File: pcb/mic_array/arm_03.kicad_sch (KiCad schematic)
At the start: 16 parts, among them U25 IM72D128V01XTMA1, U26 IM72D128V01XTMA1, U27 IM72D128V01XTMA1, U28 IM72D128V01XTMA1, U29 IM72D128V01XTMA1, U30 IM72D128V01XTMA1, U31 IM72D128V01XTMA1, U32 IM72D128V01XTMA1

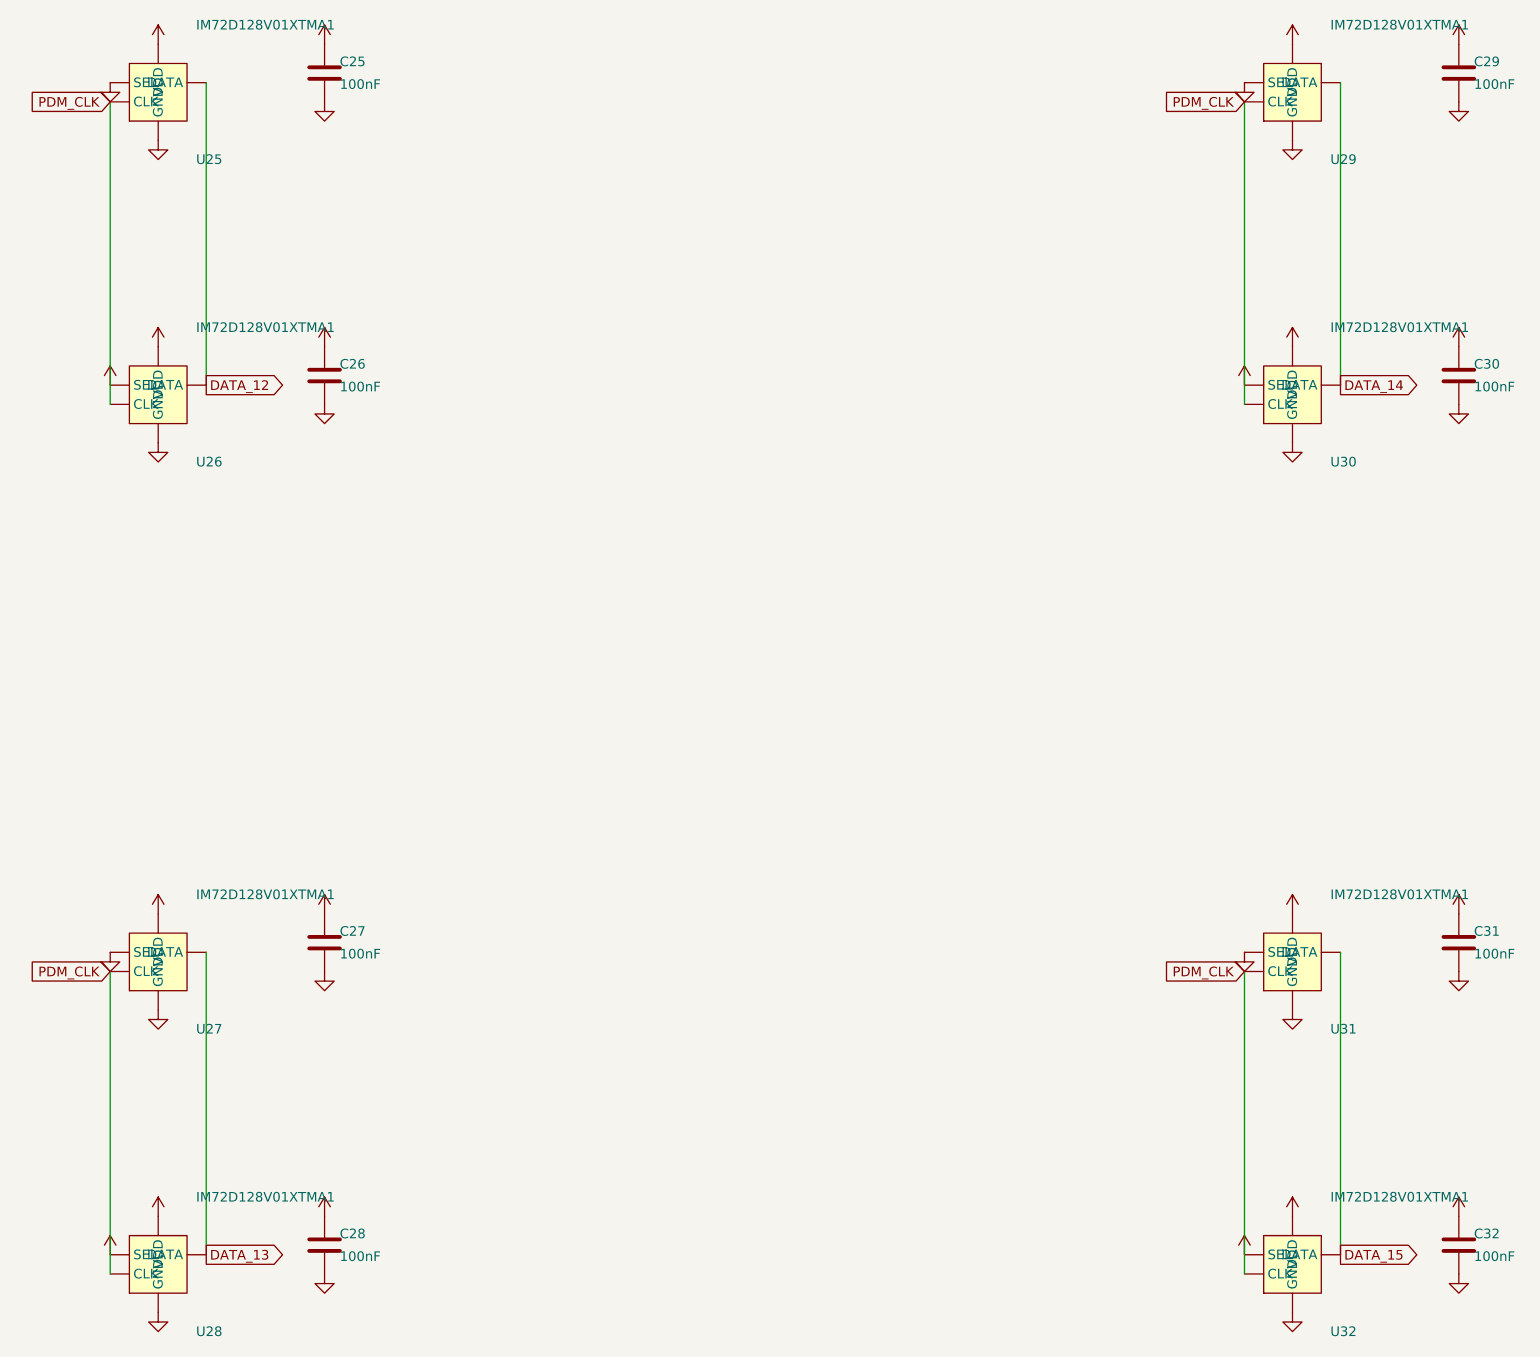
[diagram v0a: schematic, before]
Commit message: Updated.
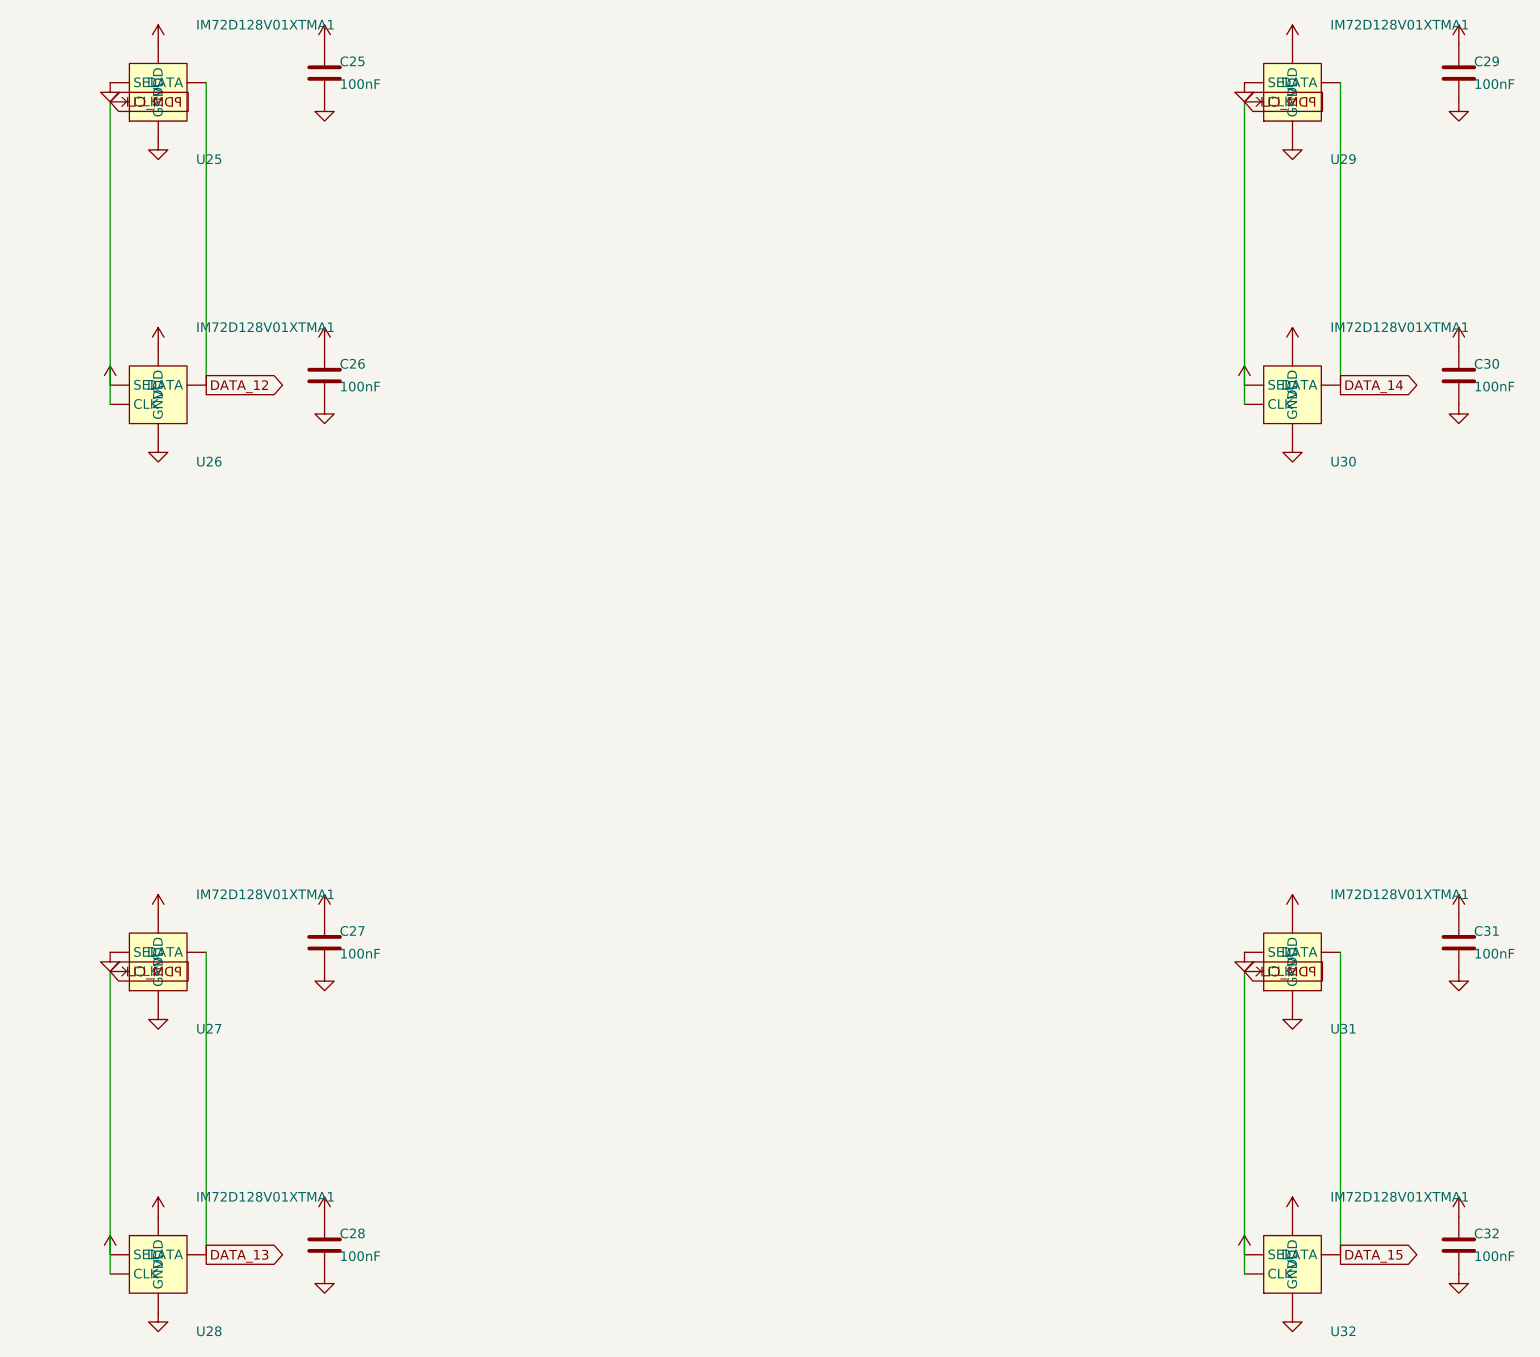
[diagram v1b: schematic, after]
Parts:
- C25, C26, C27, C28, C29, C30, C31, C32: footprint Capacitor_SMD:C_0402_1005Metric -> (none)
- U25, U26, U27, U28, U29, U30, U31, U32: footprint Sensor_Audio:Infineon_PG-LLGA-5-2 -> (none)
